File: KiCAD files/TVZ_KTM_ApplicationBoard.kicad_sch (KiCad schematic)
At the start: 64 parts, among them J1 Conn_02x19_Odd_Even, J2 Conn_02x19_Odd_Even, J3 Conn_02x19_Odd_Even, J4 Conn_02x19_Odd_Even, SW1 EG1271A, SW2 EG1271A, SW3 EG1271A, SW4 EG1271A, U1 LM75B, U2 MCP2551-I-P, U3 MCP2551-I-P

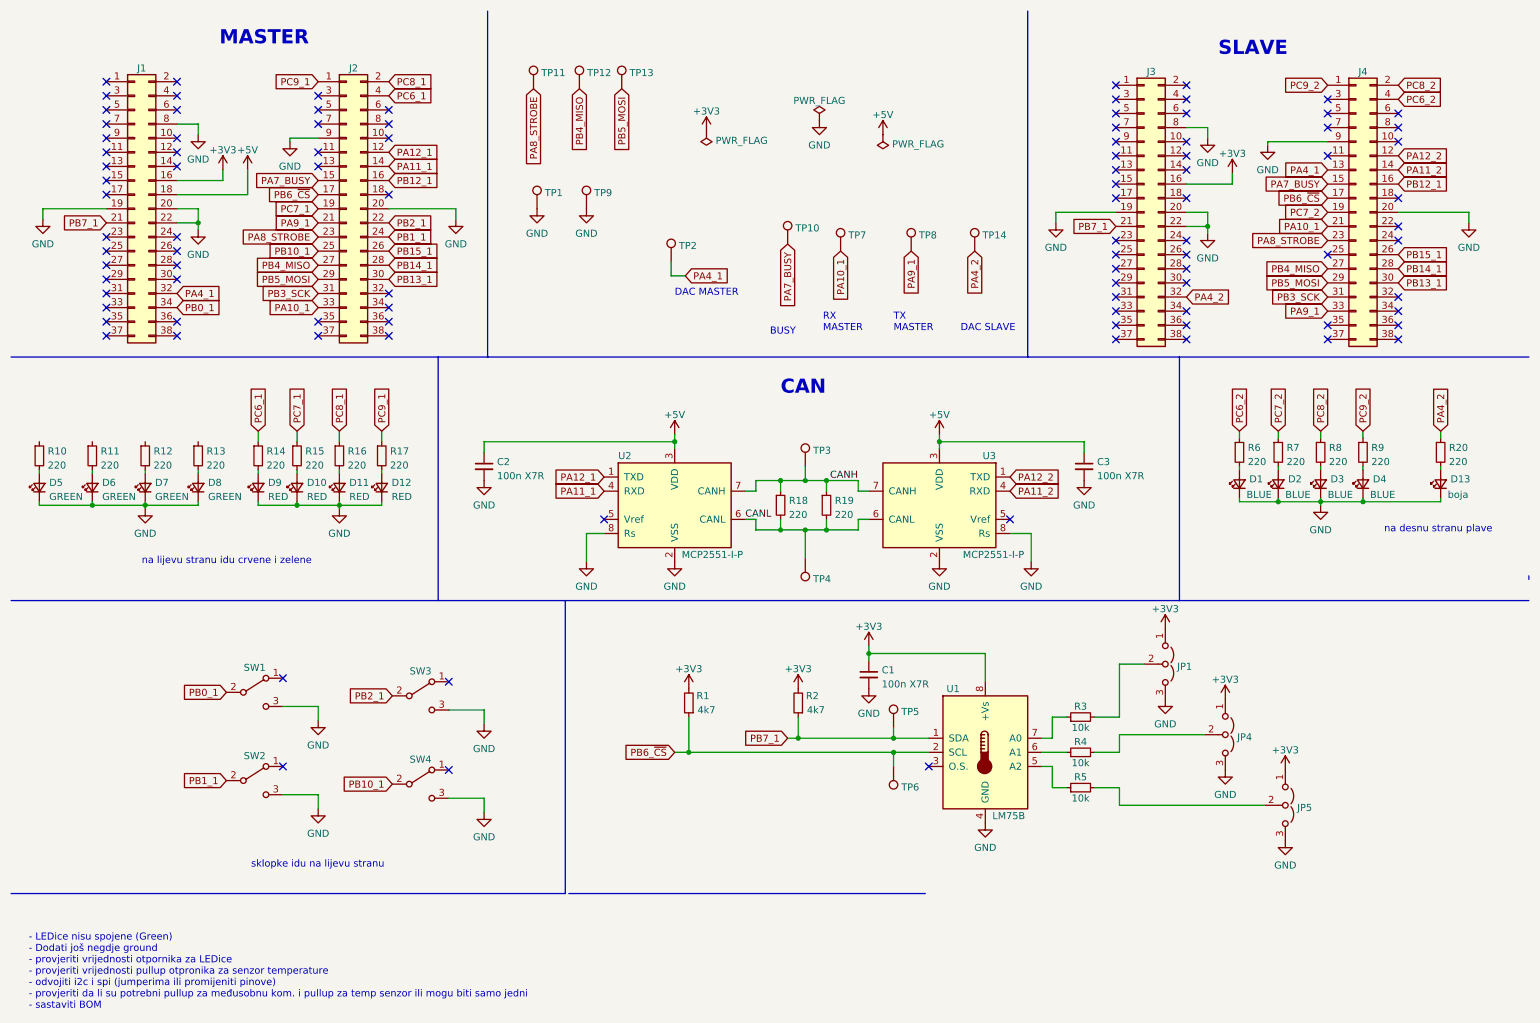
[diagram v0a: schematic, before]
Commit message: update
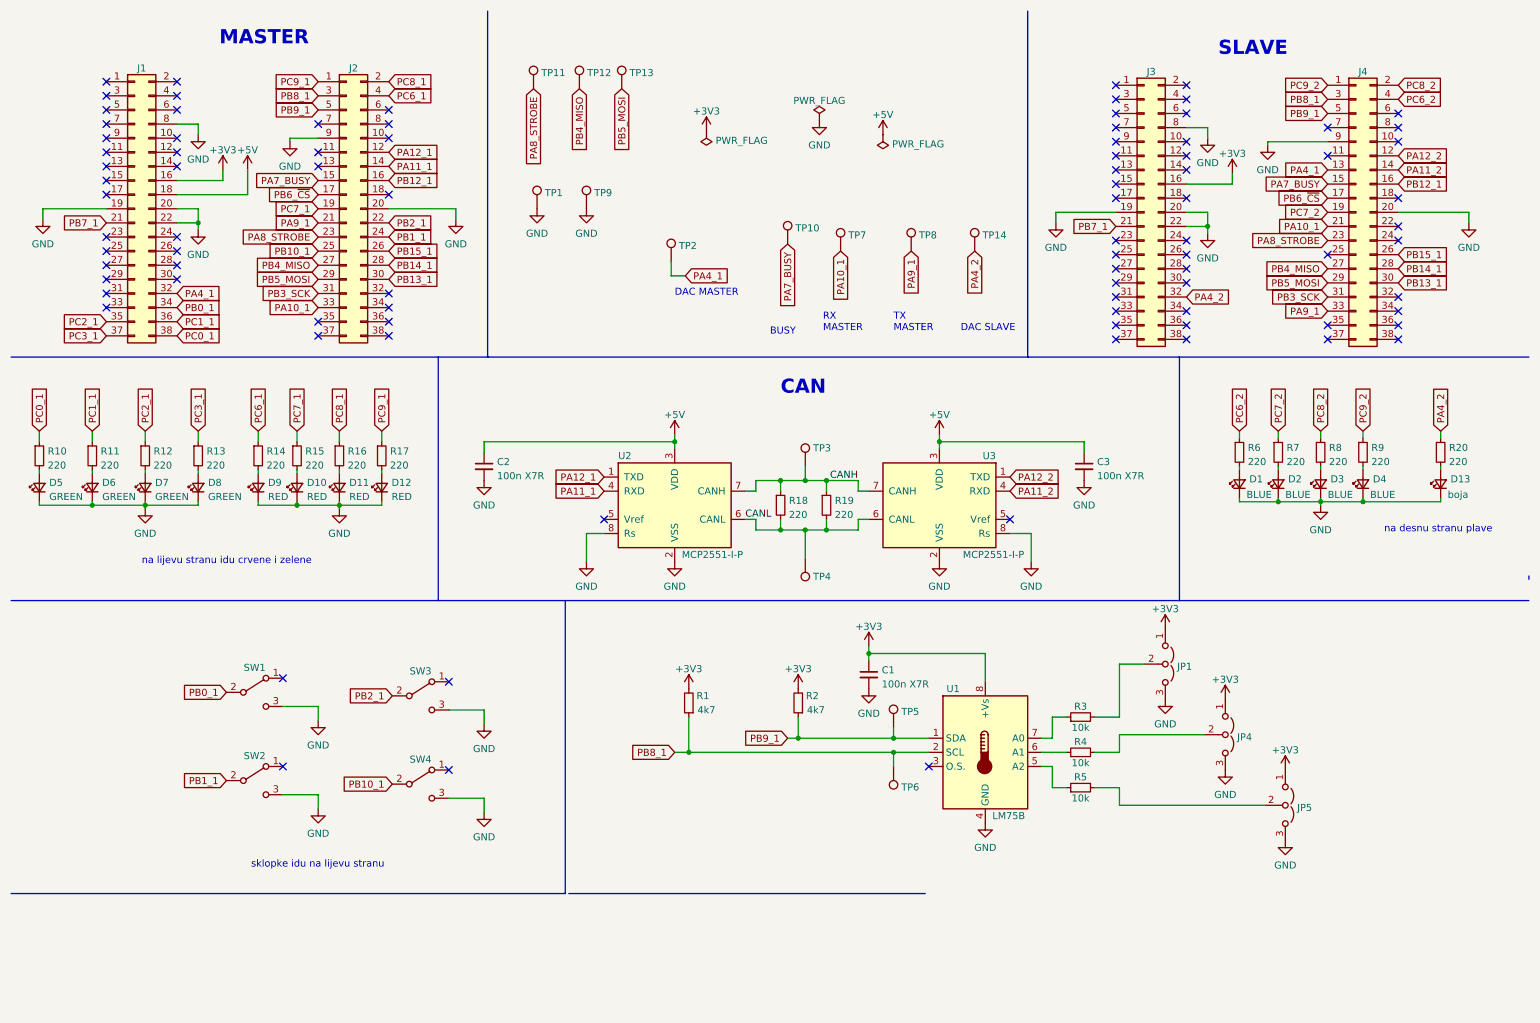
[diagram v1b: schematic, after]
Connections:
- net PB6_~{CS}: no longer R1.1, TP6.1, U1.2 (SCL)
- net PB7_1: no longer R2.1, TP5.1, U1.1 (SDA)
- net PC0_1: now reaches R10.1
- net PC0_1: now also J1.38 (Pin_38)
- net PB8_1: now reaches J4.3 (Pin_3)
- net PB8_1: now also J2.3 (Pin_3), R1.1, TP6.1, U1.2 (SCL)
- net PB9_1: now reaches J4.5 (Pin_5)
- net PB9_1: now also J2.5 (Pin_5), R2.1, TP5.1, U1.1 (SDA)
- net PC2_1: now reaches J1.35 (Pin_35)
- net PC2_1: now also R12.1
- net PC1_1: now reaches J1.36 (Pin_36)
- net PC1_1: now also R11.1
- net PC3_1: now reaches J1.37 (Pin_37)
- net PC3_1: now also R13.1
- no-connect marks 99 -> 91
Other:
- note removed: "- LEDice nisu spojene (Green) - Dodati još negdje ground - provjeriti vrijednosti otpornika za LEDice - provjeriti vrijednosti pullup otpronika za senzor temperature - odvojiti i2c i spi (jumperima ili promijeniti pinove) - provjeriti da li su potrebni pullup za međusobnu kom. i pullup za temp senzor ili mogu biti samo jedni - sastaviti BOM"
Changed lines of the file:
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@@
   (no_connect (at 67.31 32.385))
   (no_connect (at 210.82 53.34))
-  (no_connect (at 29.21 67.945))
-  (no_connect (at 67.31 27.305))
   (no_connect (at 41.91 37.465))
   (no_connect (at 67.31 70.485))
@@
   (no_connect (at 223.52 27.94))
   (no_connect (at 210.82 55.88))
-  (no_connect (at 248.92 27.94))
   (no_connect (at 223.52 35.56))
   (no_connect (at 41.91 34.925))
@@
   (no_connect (at 80.01 65.405))
   (no_connect (at 248.92 68.58))
-  (no_connect (at 248.92 30.48))
   (no_connect (at 261.62 63.5))
   (no_connect (at 223.52 60.96))
   (no_connect (at 223.52 55.88))
-  (no_connect (at 67.31 29.845))
   (no_connect (at 90.805 132.715))
   (no_connect (at 41.91 40.005))
@@
   (no_connect (at 223.52 40.64))
   (no_connect (at 248.92 33.02))
-  (no_connect (at 41.91 70.485))
   (no_connect (at 223.52 58.42))
   (no_connect (at 248.92 71.12))
@@
   (no_connect (at 29.21 27.305))
   (no_connect (at 29.21 24.765))
-  (no_connect (at 41.91 67.945))
   (no_connect (at 80.01 32.385))
   (no_connect (at 248.92 38.1))
@@
   (no_connect (at 29.21 57.785))
   (no_connect (at 191.77 103.505))
-  (no_connect (at 29.21 70.485))
   (no_connect (at 210.82 68.58))
   (no_connect (at 29.21 45.085))
@@
     (stroke (width 0) (type default))
   )
+  (wire (pts (xy 36.195 87.63) (xy 36.195 89.535))
+    (stroke (width 0) (type default))
+  )
   (wire (pts (xy 240.03 99.695) (xy 240.03 100.33))
     (stroke (width 0) (type default))
@@
     (stroke (width 0) (type default))
   )
+  (wire (pts (xy 17.145 87.63) (xy 17.145 89.535))
+    (stroke (width 0) (type default))
+  )
   (wire (pts (xy 80.01 47.625) (xy 92.075 47.625))
     (stroke (width 0) (type default))
@@
     (stroke (width 0) (type default))
   )
+  (wire (pts (xy 45.72 87.63) (xy 45.72 89.535))
+    (stroke (width 0) (type default))
+  )
   (wire (pts (xy 187.325 127.635) (xy 166.37 127.635))
     (stroke (width 0) (type default))
@@
   )
   (wire (pts (xy 67.31 34.925) (xy 62.23 34.925))
+    (stroke (width 0) (type default))
+  )
+  (wire (pts (xy 26.67 87.63) (xy 26.67 89.535))
     (stroke (width 0) (type default))
   )
@@
     (effects (font (size 1.27 1.27)) (justify left bottom))
   )
-  (text "- LEDice nisu spojene (Green)\n- Dodati još negdje ground\n- provjeriti vrijednosti otpornika za LEDice\n- provjeriti vrijednosti pullup otpronika za senzor temperature\n- odvojiti i2c i spi (jumperima ili promijeniti pinove)\n- provjeriti da li su potrebni pullup za međusobnu kom. i pullup za temp senzor ili mogu biti samo jedni\n- sastaviti BOM"
-    (at 15.24 191.77 0)
-    (effects (font (size 1.27 1.27)) (justify left bottom))
-  )
   (label "CANH" (at 159.385 96.52 0) (fields_autoplaced)
     (effects (font (size 1.27 1.27)) (justify left bottom))
@@
     )
   )
+  (global_label "PC0_1" (shape input) (at 41.91 70.485 0) (fields_autoplaced)
+    (effects (font (size 1.27 1.27)) (justify left))
+    (property "Intersheetrefs" "${INTERSHEET_REFS}" (at 50.7424 70.485 0)
+      (effects (font (size 1.27 1.27)) (justify left) hide)
+    )
+  )
   (global_label "PC7_1" (shape input) (at 63.5 87.63 90) (fields_autoplaced)
     (effects (font (size 1.27 1.27)) (justify left))
@@
     )
   )
+  (global_label "PC3_1" (shape input) (at 29.21 70.485 180) (fields_autoplaced)
+    (effects (font (size 1.27 1.27)) (justify right))
+    (property "Intersheetrefs" "${INTERSHEET_REFS}" (at 20.3776 70.485 0)
+      (effects (font (size 1.27 1.27)) (justify right) hide)
+    )
+  )
+  (global_label "PB9_1" (shape input) (at 151.765 142.875 180) (fields_autoplaced)
+    (effects (font (size 1.27 1.27)) (justify right))
+    (property "Intersheetrefs" "${INTERSHEET_REFS}" (at 142.9326 142.875 0)
+      (effects (font (size 1.27 1.27)) (justify right) hide)
+    )
+  )
+  (global_label "PB9_1" (shape input) (at 248.92 30.48 180) (fields_autoplaced)
+    (effects (font (size 1.27 1.27)) (justify right))
+    (property "Intersheetrefs" "${INTERSHEET_REFS}" (at 240.0876 30.48 0)
+      (effects (font (size 1.27 1.27)) (justify right) hide)
+    )
+  )
   (global_label "PB14_1" (shape input) (at 80.01 57.785 0) (fields_autoplaced)
     (effects (font (size 1.27 1.27)) (justify left))
@@
     )
   )
-  (global_label "PB7_1" (shape input) (at 151.765 142.875 180) (fields_autoplaced)
-    (effects (font (size 1.27 1.27)) (justify right))
-    (property "Intersheetrefs" "${INTERSHEET_REFS}" (at 143.4252 142.7956 0)
-      (effects (font (size 1.27 1.27)) (justify right) hide)
+  (global_label "PC1_1" (shape input) (at 26.67 87.63 90) (fields_autoplaced)
+    (effects (font (size 1.27 1.27)) (justify left))
+    (property "Intersheetrefs" "${INTERSHEET_REFS}" (at 26.67 78.7976 90)
+      (effects (font (size 1.27 1.27)) (justify left) hide)
     )
   )
@@
     )
   )
+  (global_label "PB8_1" (shape input) (at 248.92 27.94 180) (fields_autoplaced)
+    (effects (font (size 1.27 1.27)) (justify right))
+    (property "Intersheetrefs" "${INTERSHEET_REFS}" (at 240.0876 27.94 0)
+      (effects (font (size 1.27 1.27)) (justify right) hide)
+    )
+  )
   (global_label "PB5_MOSI" (shape input) (at 121.92 26.035 270) (fields_autoplaced)
     (effects (font (size 1.27 1.27)) (justify right))
@@
     )
   )
+  (global_label "PC0_1" (shape input) (at 17.145 87.63 90) (fields_autoplaced)
+    (effects (font (size 1.27 1.27)) (justify left))
+    (property "Intersheetrefs" "${INTERSHEET_REFS}" (at 17.145 78.7976 90)
+      (effects (font (size 1.27 1.27)) (justify left) hide)
+    )
+  )
   (global_label "PB7_1" (shape input) (at 29.21 50.165 180) (fields_autoplaced)
     (effects (font (size 1.27 1.27)) (justify right))
@@
     )
   )
+  (global_label "PC3_1" (shape input) (at 45.72 87.63 90) (fields_autoplaced)
+    (effects (font (size 1.27 1.27)) (justify left))
+    (property "Intersheetrefs" "${INTERSHEET_REFS}" (at 45.72 78.7976 90)
+      (effects (font (size 1.27 1.27)) (justify left) hide)
+    )
+  )
   (global_label "PA12_1" (shape input) (at 118.745 95.885 180) (fields_autoplaced)
     (effects (font (size 1.27 1.27)) (justify right))
@@
     )
   )
+  (global_label "PC1_1" (shape input) (at 41.91 67.945 0) (fields_autoplaced)
+    (effects (font (size 1.27 1.27)) (justify left))
+    (property "Intersheetrefs" "${INTERSHEET_REFS}" (at 50.7424 67.945 0)
+      (effects (font (size 1.27 1.27)) (justify left) hide)
+    )
+  )
   (global_label "PC9_2" (shape input) (at 255.27 87.63 90) (fields_autoplaced)
     (effects (font (size 1.27 1.27)) (justify left))
@@
     )
   )
+  (global_label "PC2_1" (shape input) (at 36.195 87.63 90) (fields_autoplaced)
+    (effects (font (size 1.27 1.27)) (justify left))
+    (property "Intersheetrefs" "${INTERSHEET_REFS}" (at 36.195 78.7976 90)
+      (effects (font (size 1.27 1.27)) (justify left) hide)
+    )
+  )
   (global_label "PA4_1" (shape input) (at 133.35 59.69 0) (fields_autoplaced)
     (effects (font (size 1.27 1.27)) (justify left))
@@
     )
   )
-  (global_label "PB6_~{CS}" (shape input) (at 131.445 145.415 180) (fields_autoplaced)
-    (effects (font (size 1.27 1.27)) (justify right))
-    (property "Intersheetrefs" "${INTERSHEET_REFS}" (at 121.8352 145.3356 0)
+  (global_label "PB8_1" (shape input) (at 131.445 145.415 180) (fields_autoplaced)
+    (effects (font (size 1.27 1.27)) (justify right))
+    (property "Intersheetrefs" "${INTERSHEET_REFS}" (at 122.6126 145.415 0)
       (effects (font (size 1.27 1.27)) (justify right) hide)
     )
@@
     )
   )
+  (global_label "PC2_1" (shape input) (at 29.21 67.945 180) (fields_autoplaced)
+    (effects (font (size 1.27 1.27)) (justify right))
+    (property "Intersheetrefs" "${INTERSHEET_REFS}" (at 20.3776 67.945 0)
+      (effects (font (size 1.27 1.27)) (justify right) hide)
+    )
+  )
   (global_label "PA7_BUSY" (shape input) (at 151.765 53.975 270) (fields_autoplaced)
     (effects (font (size 1.27 1.27)) (justify right))
@@
     )
   )
+  (global_label "PB8_1" (shape input) (at 67.31 27.305 180) (fields_autoplaced)
+    (effects (font (size 1.27 1.27)) (justify right))
+    (property "Intersheetrefs" "${INTERSHEET_REFS}" (at 58.4776 27.305 0)
+      (effects (font (size 1.27 1.27)) (justify right) hide)
+    )
+  )
   (global_label "PC7_2" (shape input) (at 248.92 48.26 180) (fields_autoplaced)
     (effects (font (size 1.27 1.27)) (justify right))
@@
     (effects (font (size 1.27 1.27)) (justify right))
     (property "Intersheetrefs" "${INTERSHEET_REFS}" (at 237.1936 60.8806 0)
+      (effects (font (size 1.27 1.27)) (justify right) hide)
+    )
+  )
+  (global_label "PB9_1" (shape input) (at 67.31 29.845 180) (fields_autoplaced)
+    (effects (font (size 1.27 1.27)) (justify right))
+    (property "Intersheetrefs" "${INTERSHEET_REFS}" (at 58.4776 29.845 0)
       (effects (font (size 1.27 1.27)) (justify right) hide)
     )
@@
   (symbol (lib_id "Connector:TestPoint") (at 154.94 93.98 0) (unit 1)
     (in_bom yes) (on_board yes) (dnp no) (fields_autoplaced)
-    (property "Reference" "TP3" (at 156.337 91.1118 0)
+    (property "Reference" "TP3" (at 156.337 90.678 0)
       (effects (font (size 1.27 1.27)) (justify left))
     )
@@
   (symbol (lib_id "Connector:TestPoint") (at 154.94 110.49 180) (unit 1)
     (in_bom yes) (on_board yes) (dnp no) (fields_autoplaced)
-    (property "Reference" "TP4" (at 156.337 114.2258 0)
+    (property "Reference" "TP4" (at 156.337 113.792 0)
       (effects (font (size 1.27 1.27)) (justify right))
     )
